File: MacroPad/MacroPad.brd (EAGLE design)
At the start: 120.6 x 69.5 mm, 70 parts, among them IC1 MIC5219BM5, J1 USB4085-GF-A_REVA4, U1 ATMEGA32U4-AUR, Y1 XRCGB16M000FXN00R0

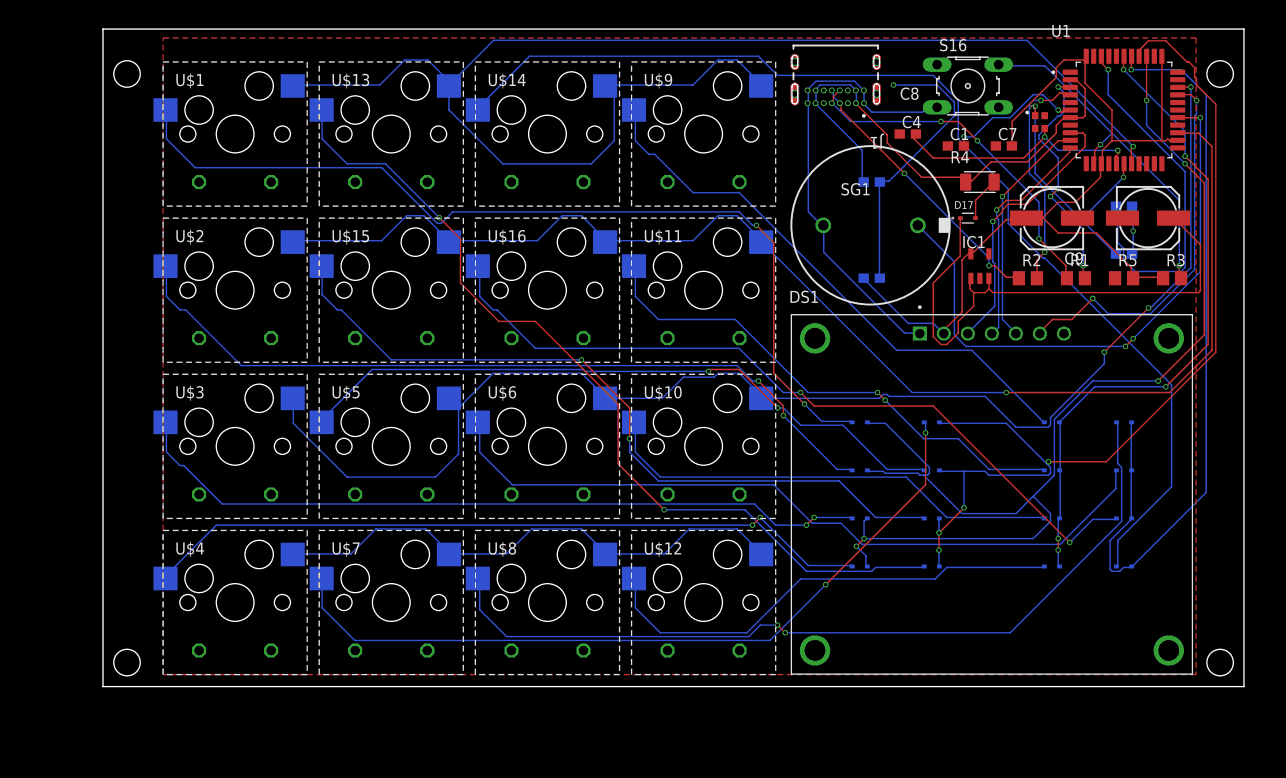
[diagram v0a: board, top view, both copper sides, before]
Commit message: Further board errors corrected, BOM included
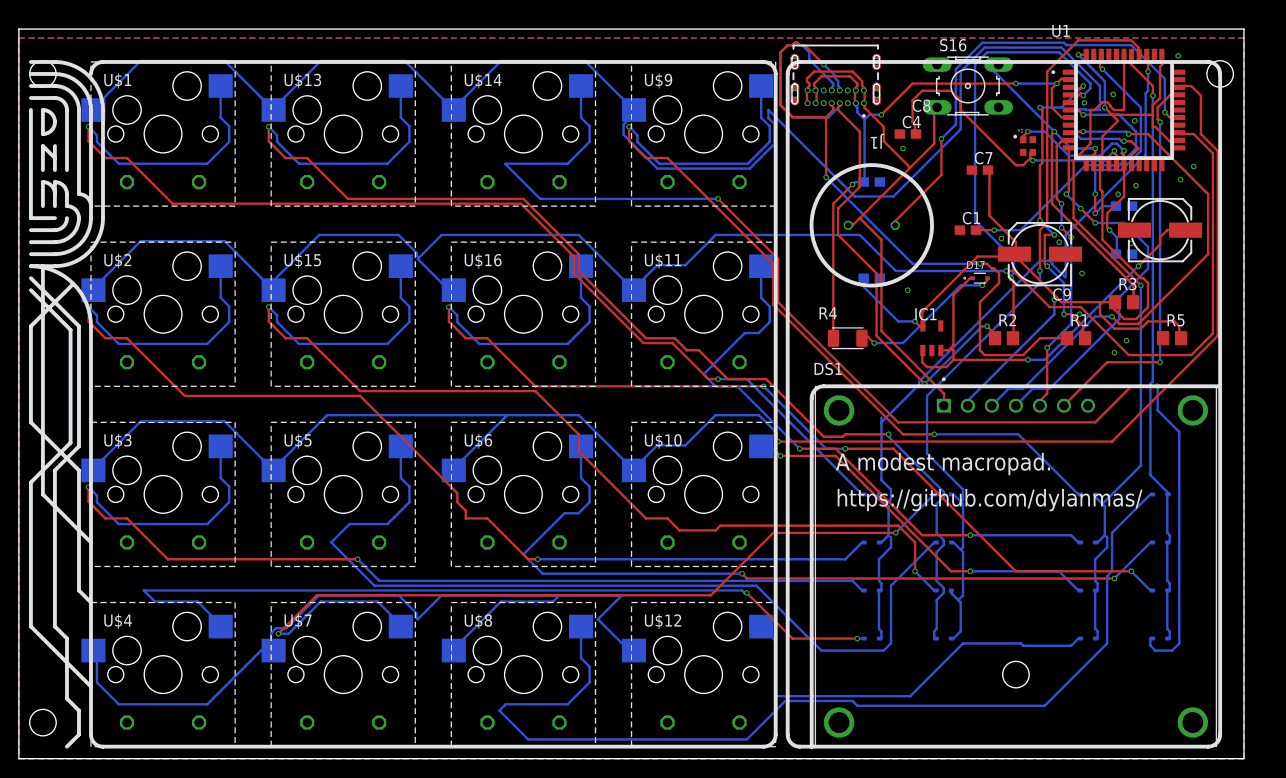
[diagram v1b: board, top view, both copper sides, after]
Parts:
- removed SG1: EFBAA40D101, buzzer:EFBAA40D101
- added U$17: PT-1307, PT-1307:PT-1307
- moved R4 21.6 mm to (78.7, 36.8)
- moved U$4 10.8 mm to (6.35, 1.27)
- moved S5 10.8 mm to (5.71, 5.08), turned to 180 degrees
- moved IC1 9.16 mm to (87.6, 36.8)
- moved S2 9.16 mm to (5.71, 24.1), turned to 180 degrees
- moved U$7 9.16 mm to (25.4, 1.27)
- moved U$3 9.16 mm to (6.35, 20.3)
- moved S7 9.16 mm to (24.8, 5.08), turned to 180 degrees
- moved C1 8.98 mm to (91.4, 48.3)
- moved D10 8.52 mm to (104.1, 15.2)
- moved D11 8.52 mm to (104.1, 10.2)
- moved D12 8.52 mm to (104.1, 5.08)
- moved D13 8.52 mm to (111.8, 20.3)
- moved D14 8.52 mm to (111.8, 15.2)
- moved D15 8.52 mm to (111.8, 10.2)
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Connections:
- net D7: now also U$17.P$2; no longer SG1.2
- net DGND: now also U$17.P$1; no longer SG1.1
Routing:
- net N$21: track 29.2 -> 68.6 mm
- net N$5: track 92.3 -> 131.2 mm
- net A0: track 120.6 -> 82.6 mm, vias 5 -> 1
- net N$2: track 83.9 -> 119.9 mm
- net GND: track 34.9 -> 0.00 mm, vias 2 -> 17
- net D6: track 56.8 -> 91.0 mm
- net N$20: track 37.2 -> 70.3 mm
- net N$13: track 59.0 -> 91.4 mm, vias 0 -> 2
- net N$3: track 79.3 -> 111.6 mm
- net N$6: track 79.2 -> 111.3 mm
- net D5: track 144.2 -> 174.2 mm, vias 3 -> 1
- net D4: track 138.7 -> 168.1 mm
- net N$10: track 82.5 -> 111.8 mm, vias 2 -> 4
- net VCC: track 100.6 -> 127.8 mm, vias 0 -> 4
- net N$1: track 97.2 -> 124.2 mm
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- added copper zone on layer 16, net GND
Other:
- board size 120.6 x 69.5 mm -> 129.5 x 77.1 mm
- board text added: "A modest macropad."
- board text added: "https://github.com/dylanmas/"
- board text removed: "Dyl's Macropad"
- board text removed: "If you're reading this: have a nice day!"
